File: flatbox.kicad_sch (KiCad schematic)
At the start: 39 parts, among them J3 USB_C_Receptacle_USB2.0_16P, SW1 SW_Push, SW10 SW_Push, SW11 SW_Push, SW12 SW_Push, SW13 SW_Push, SW2 SW_Push, SW3 SW_Push, SW4 SW_Push, SW5 SW_Push, SW6 SW_Push, SW7 SW_Push, SW8 SW_Push, SW9 SW_Push, U1 ATmega32U4-A, Y1 16MHz

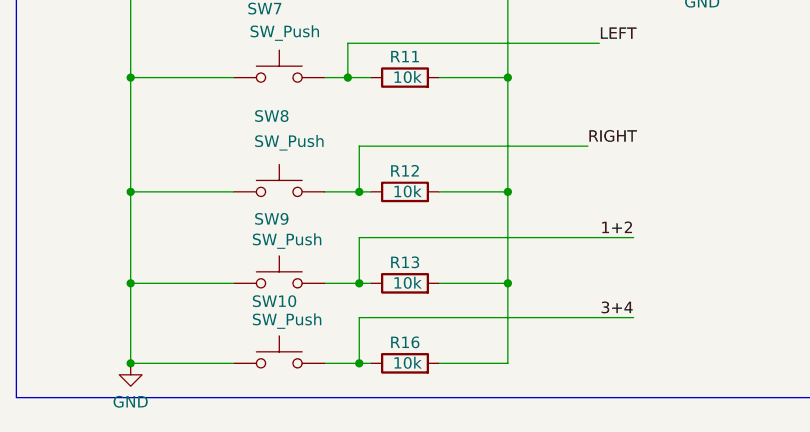
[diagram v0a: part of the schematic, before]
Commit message: Updated PCB & Schematic
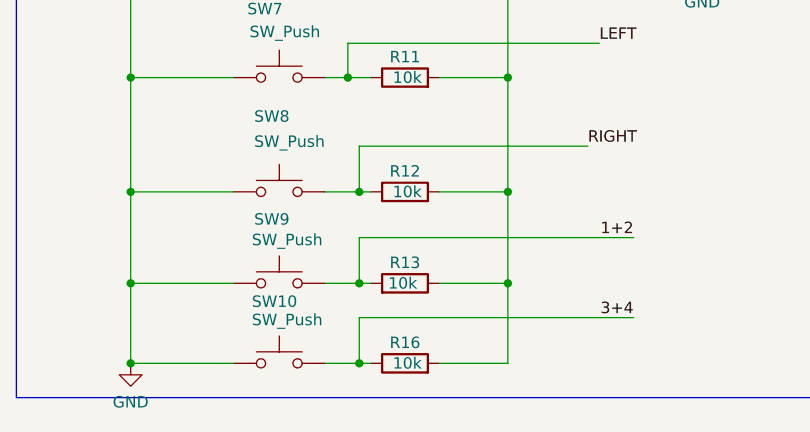
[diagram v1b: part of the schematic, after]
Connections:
- net +5V: now also R13.1; no longer R13.2
- net 1+2: now also R13.2; no longer R13.1
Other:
- moved on the sheet: R13
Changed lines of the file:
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@@
 	(symbol
 		(lib_id "Device:R")
-		(at 55.88 184.15 90)
+		(at 55.88 184.15 270)
+		(mirror x)
 		(unit 1)
 		(body_style 1)
@@
 		)
 		(property "Value" "10k"
-			(at 56.134 184.15 90)
+			(at 55.626 184.15 90)
 			(show_name no)
 			(do_not_autoplace no)
